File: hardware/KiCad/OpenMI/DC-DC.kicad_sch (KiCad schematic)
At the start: 37 parts, among them Q4 GAN7R0-150LBEZ, Q5 GAN7R0-150LBEZ, U3 1EDN7550B, U4 1EDN7550B

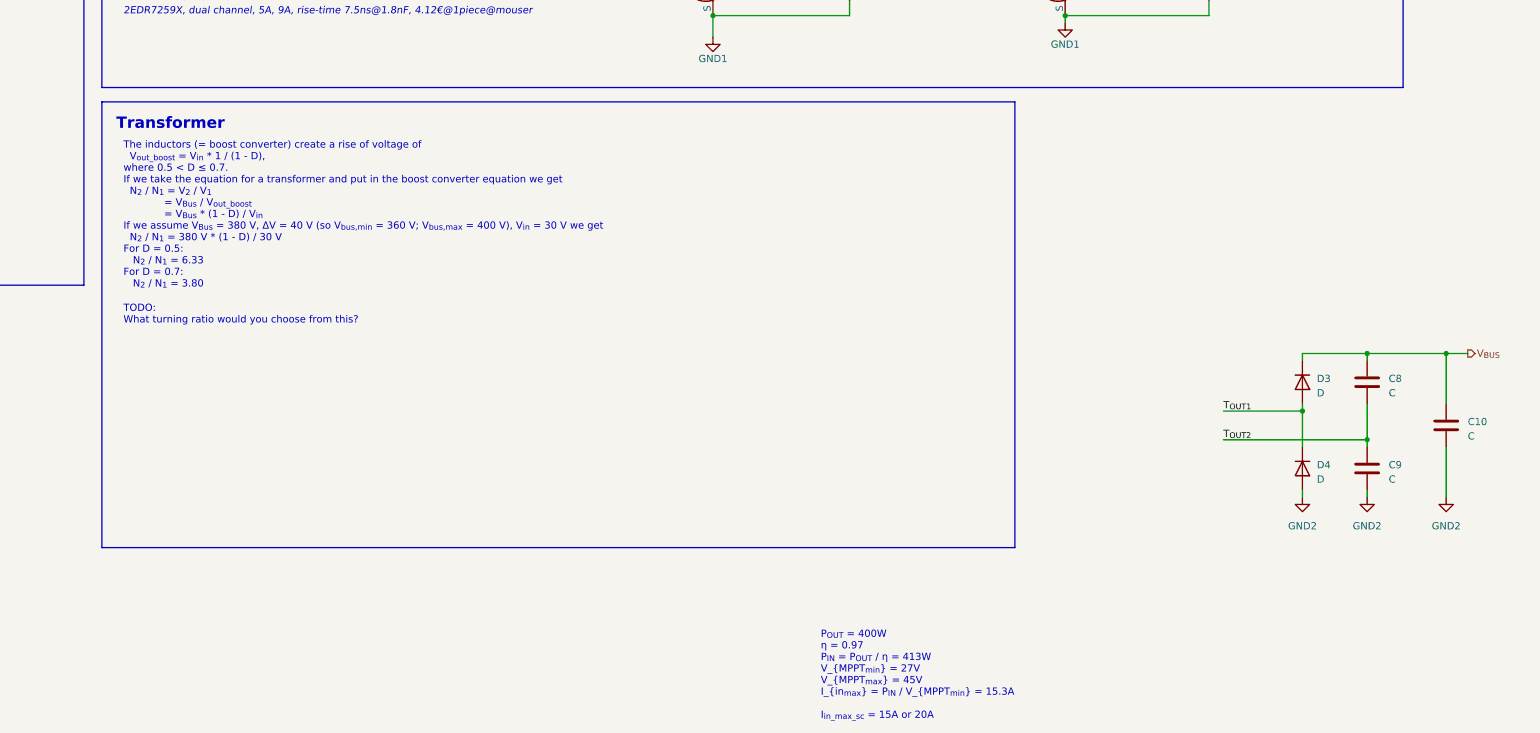
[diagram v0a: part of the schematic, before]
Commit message: feat: adds first considerations about rectifier
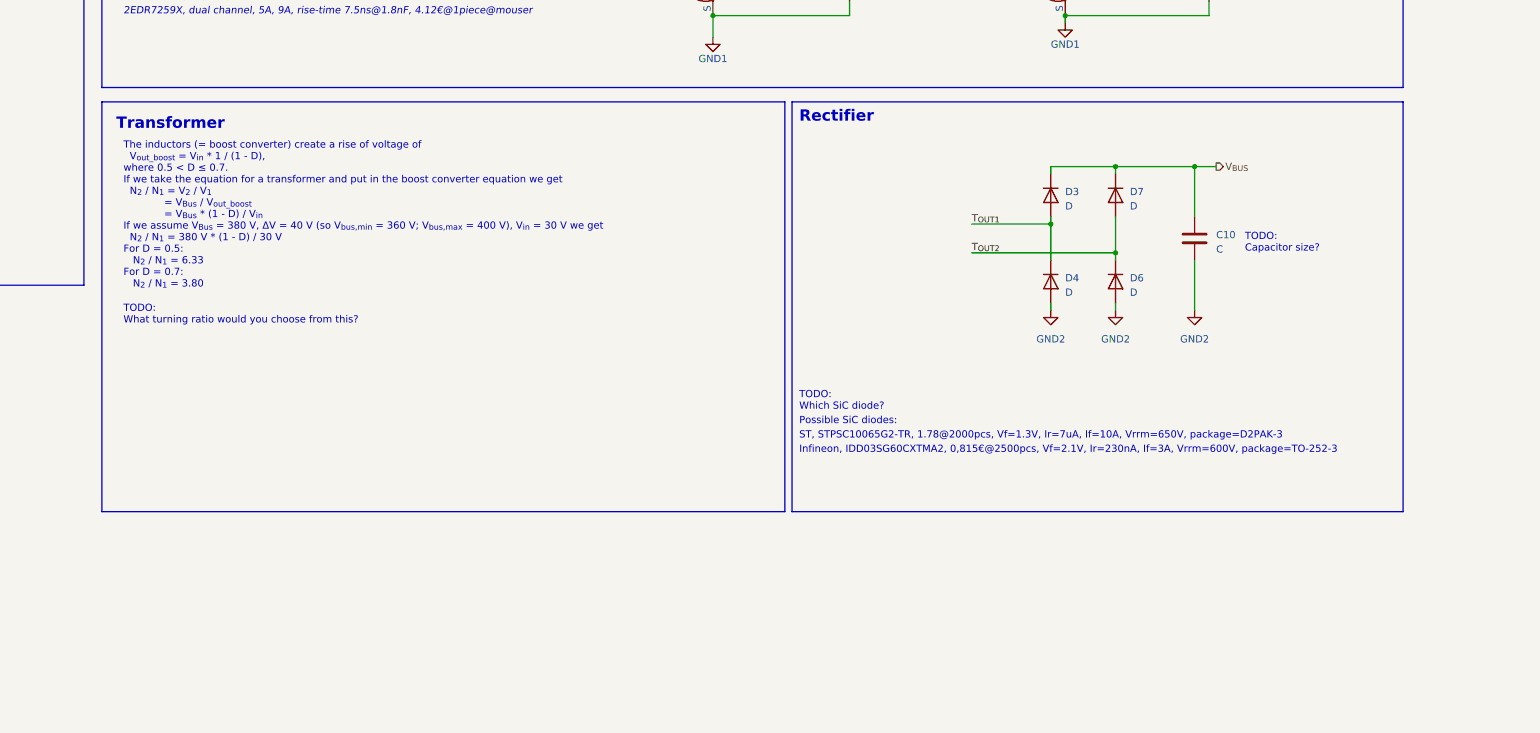
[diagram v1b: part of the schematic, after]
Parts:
- removed C8, C9: C, symbol Device:C
- added D6, D7: D, symbol Device:D
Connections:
- net GND2: now also D6.2 (A)
- net T_{OUT2}: now also D6.1 (K), D7.2 (A)
- net V_{BUS}: now also D7.1 (K)
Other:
- note added: "Infineon, IDD03SG60CXTMA2, 0,815€@2500pcs, Vf=2.1V, Ir=230nA, If=3A, Vrrm=600V, package=TO-252-3"
- note added: "Possible SiC diodes:"
- note added: "Rectifier"
- note added: "ST, STPSC10065G2-TR, 1.78@2000pcs, Vf=1.3V, Ir=7uA, If=10A, Vrrm=650V, package=D2PAK-3"
- note added: "TODO: Capacitor size?"
- note added: "TODO: Which SiC diode?"
- note removed: "P_{OUT} = 400W η = 0.97 P_{IN} = P_{OUT} / η = 413W V_{MPPT_{min}} = 27V V_{MPPT_{max}} = 45V I_{in_{max}} = P_{IN} / V_{MPPT_{min}} = 15.3A I_{in_max_sc} = 15A or 20A"
- moved on the sheet: C10, D3, D4
